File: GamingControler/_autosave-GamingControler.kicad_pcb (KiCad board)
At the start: 2 copper layers, 53 x 63 mm, 52 parts, among them J1 USB_C_Receptacle_USB2.0_16P, J2 USB_C_Receptacle_USB2.0_16P, J3 Conn_01x05_Pin, J4 Conn_01x05_Pin, SW1 SW_Push, SW2 SW_Push, U1 ESP32-C6-WROOM-1, U2 AZ1117-3.3, U3 CP2102N-Axx-xQFN20, U4 TTP223-BA6, U5 TTP223-BA6, U6 TTP223-BA6, U7 TTP223-BA6

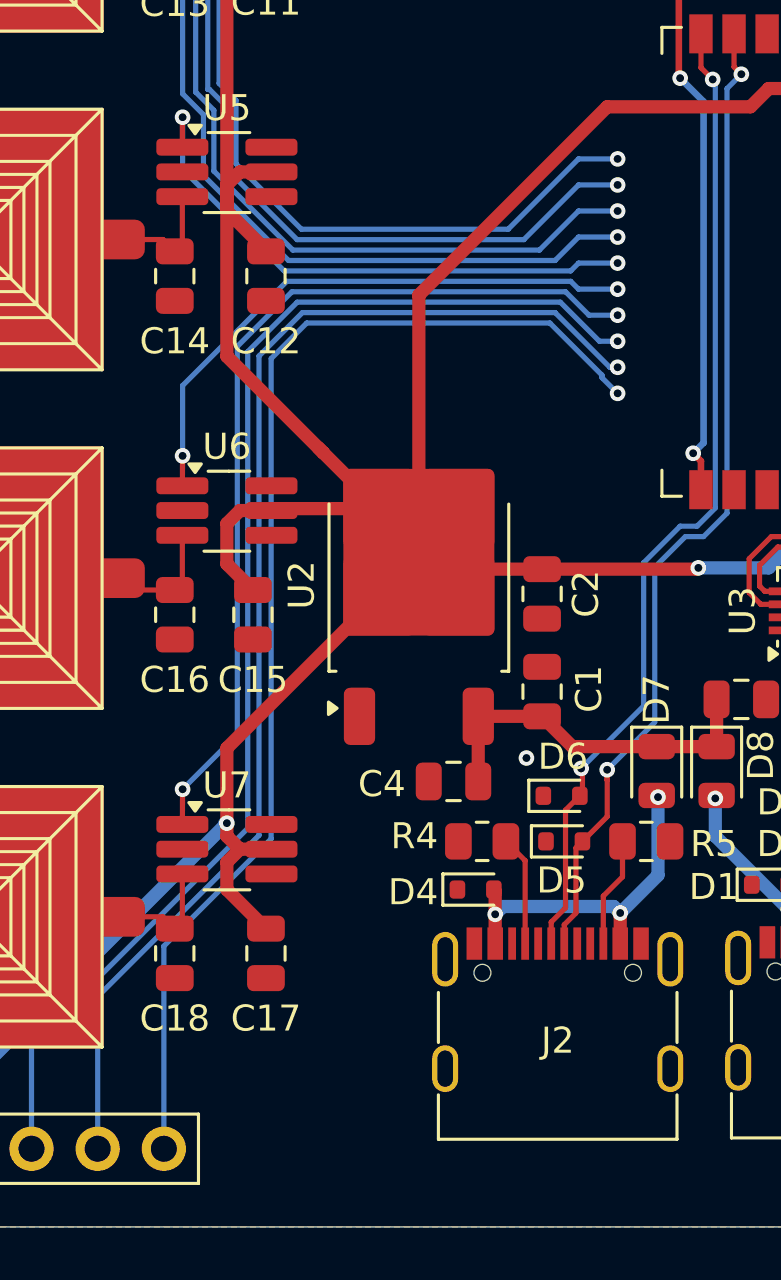
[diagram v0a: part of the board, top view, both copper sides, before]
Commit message: summary
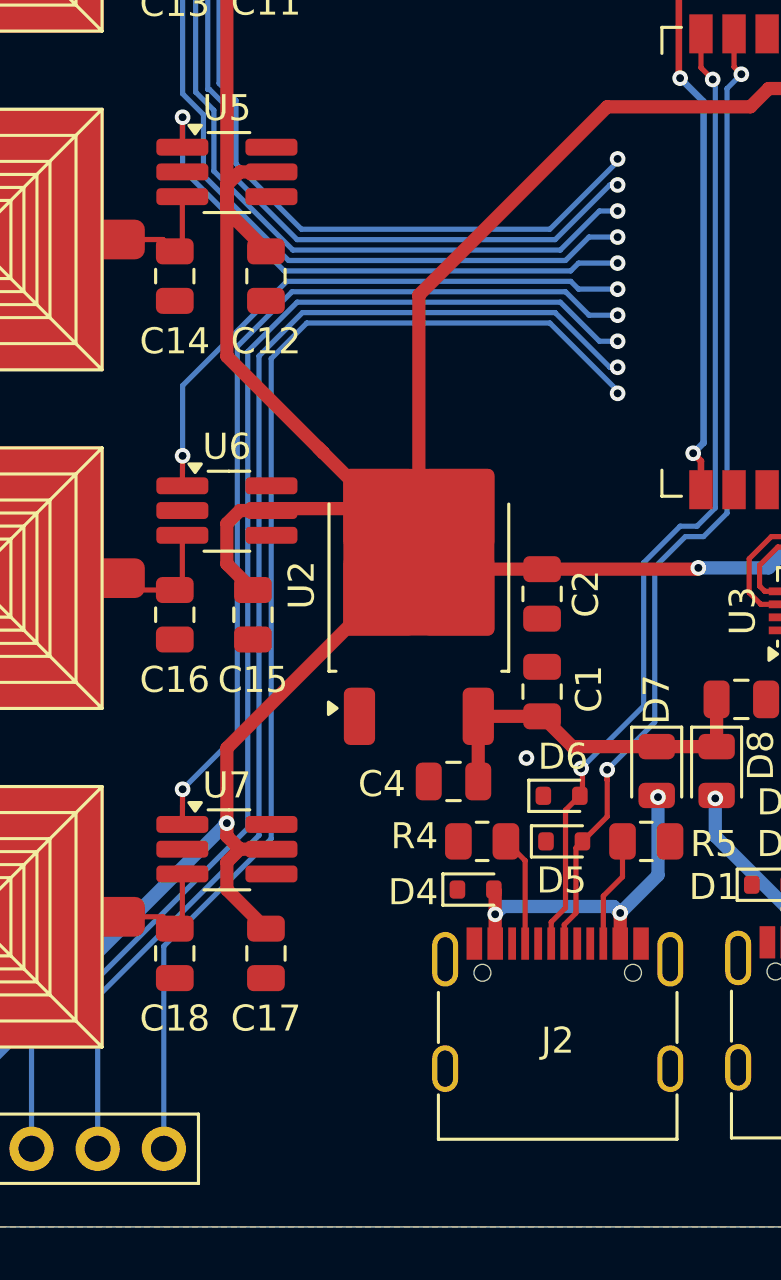
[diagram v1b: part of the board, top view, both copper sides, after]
